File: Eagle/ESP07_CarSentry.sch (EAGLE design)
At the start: 45 parts, among them Q1 PFET, Q2 NPN or N-FET, Q3 PFET, Q4 NPN

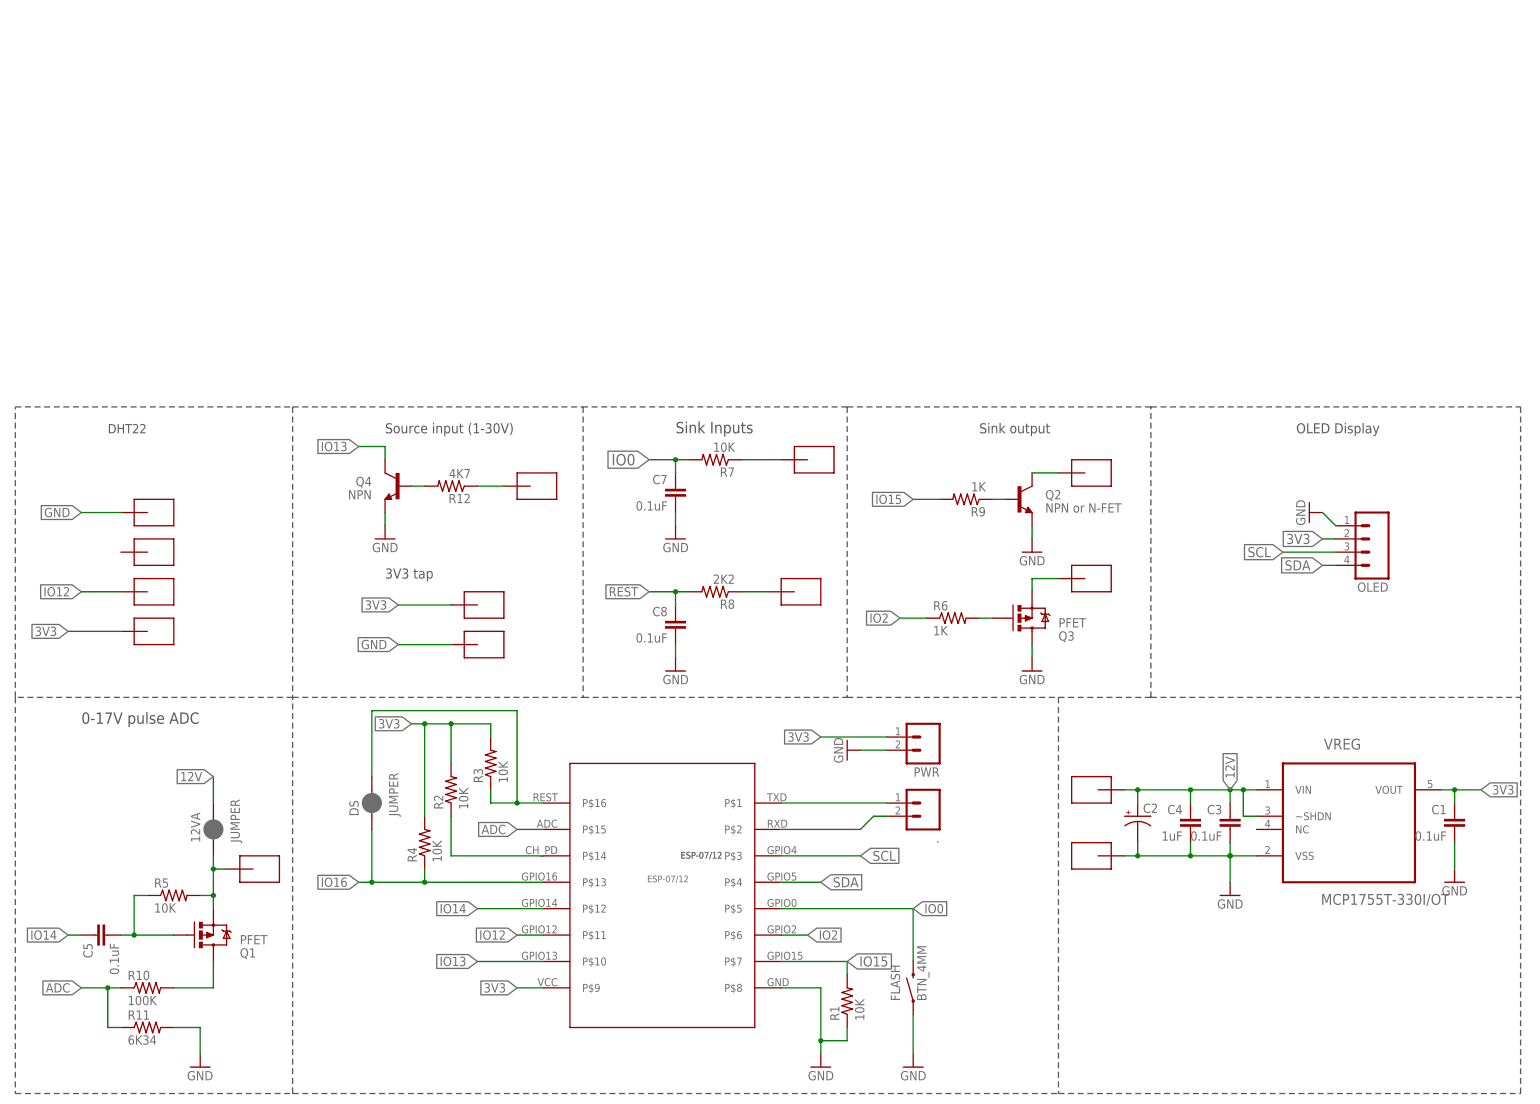
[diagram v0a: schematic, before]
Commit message: rev 3
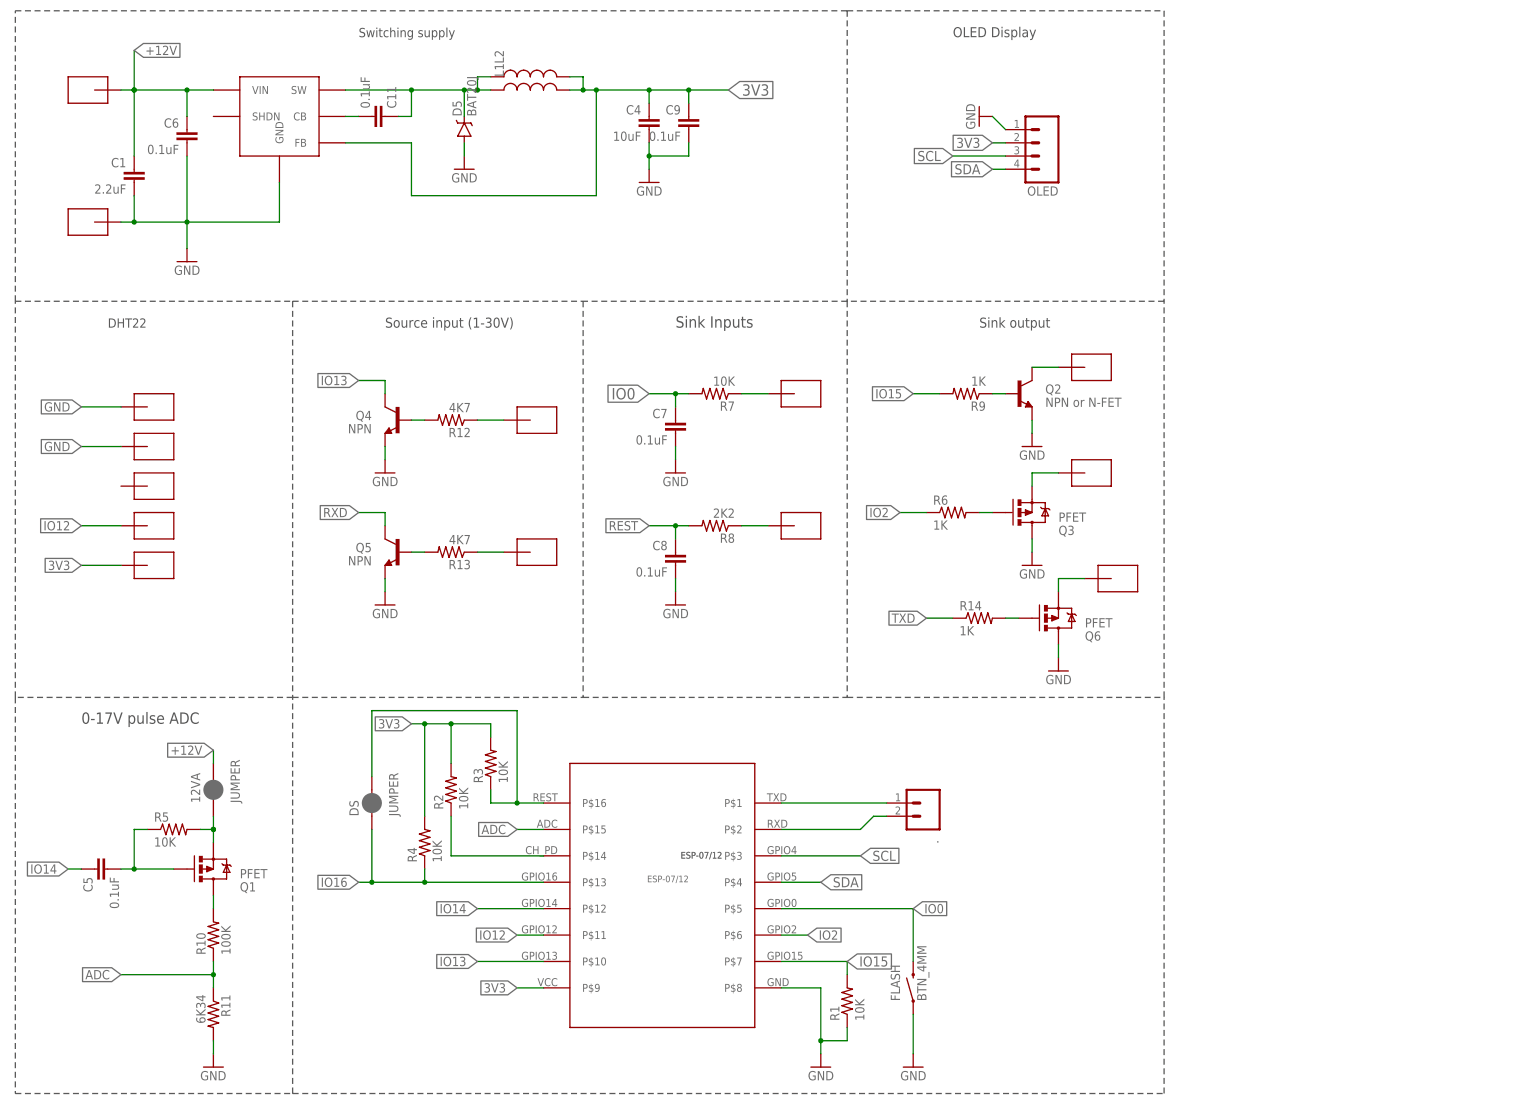
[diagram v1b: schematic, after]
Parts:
- removed C2: (no value), SparkFun-Capacitors:CAP_POLPTH1
- removed C3: 0.1uF, SparkFun-Capacitors:CAP
- removed PWR: (no value), SparkFun-Connectors:M02PTH
- removed VREG: MCP1755T-330I/OT, Microchip_By_element14_Batch_1:MCP1802T-3002I/OT
- added C11, C6, C9: 0.1uF, SparkFun-Capacitors:CAP
- added D5: BAT20J, SparkFun-DiscreteSemi:DIODE-SCHOTTKY-BAT20J
- added L1, L2: (no value), SparkFun-Passives:INDUCTOR0805
- added Q5: NPN, SparkFun-DiscreteSemi:TRANSISTOR_NPNSOT23-3
- added Q6: PFET, SparkFun-DiscreteSemi:MOSFET-PCHANNEL
- added R13: 4K7, SparkFun-Resistors:RESISTOR0805-RES
- added R14: 1K, SparkFun-Resistors:RESISTOR0805-RES
- added VREG1: LMR16006YQ3DDCRQ1, CuriousTech:LMR16006YQ
- C1: value 0.1uF -> 2.2uF
- C4: value 1uF -> 10uF
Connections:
- removed net 12V: 12VA.2, C2.+, C3.1, C4.1, U$16.P$1, VREG.VIN, VREG.~SHDN
- new net +12V: 12VA.2, C1.1, C6.1, U$16.P$1, VREG1.VIN
- new net N$12: Q5.B, R13.2
- new net N$13: C11.1, D5.C, L1.1, L2.1, VREG1.SW
- new net N$14: C11.2, VREG1.CB
- new net N$15: R13.1, U$10.P$1
- new net N$16: Q6.S, U$13.P$1
- new net N$17: Q6.G, R14.2
- net 3V3: now also C4.1, C9.1, L1.2, L2.2, VREG1.FB; no longer C1.1, PWR.1, U$10.P$1, VREG.VOUT
- net ADCHI: no longer U$13.P$1
- net GND: now also C6.2, C9.2, D5.A, Q5.E, Q6.D, VREG1.GND; no longer C2.-, C3.2, PWR.2, VREG.VSS
- net RXD: now also Q5.C
- net TXD: now also R14.1
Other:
- note added: "Switching supply"
- note removed: "3V3 tap"
- moved on the sheet: 12VA, C1, C4, C5, C7, C8, OLED, Q1, Q2, Q3, Q4, R10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
